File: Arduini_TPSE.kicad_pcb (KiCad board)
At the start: 2 copper layers, 26 x 57.5 mm, 27 parts, among them J1 2134441-2, J2 ICSP, P1 Digital, P2 Analog, SW1 SW_Push, U1 AMS1117-5.0, U2 FT232RL, U3 ATmega328-P, U4 AMS1117-3.3, Y1 16Mhz

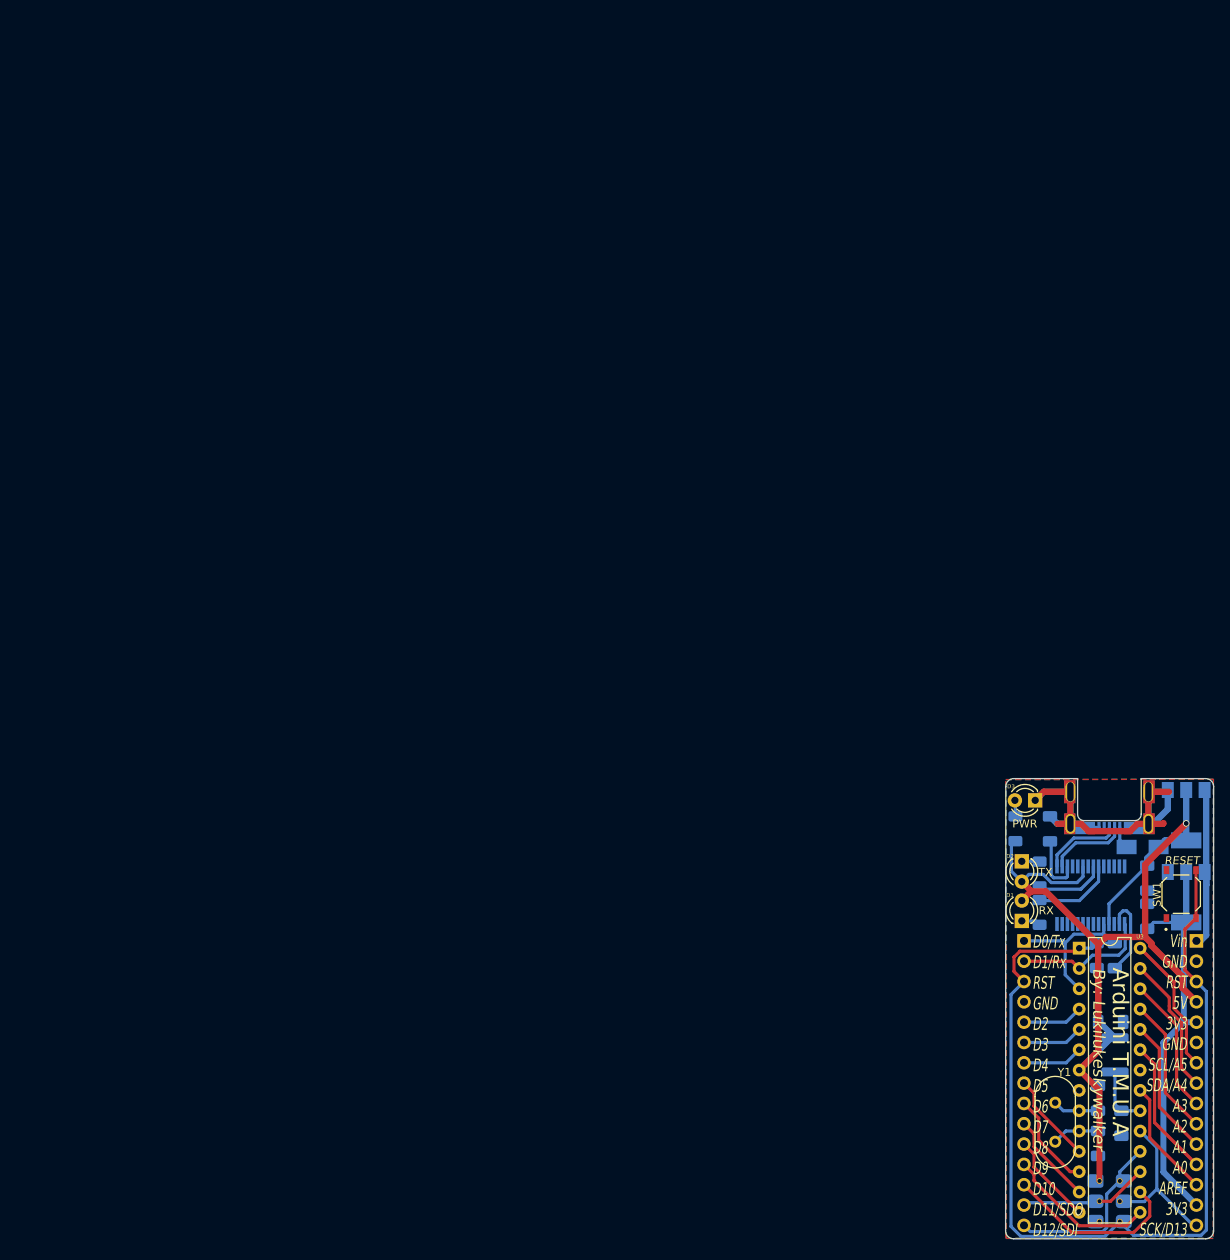
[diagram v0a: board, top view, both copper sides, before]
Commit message: Ampliacion
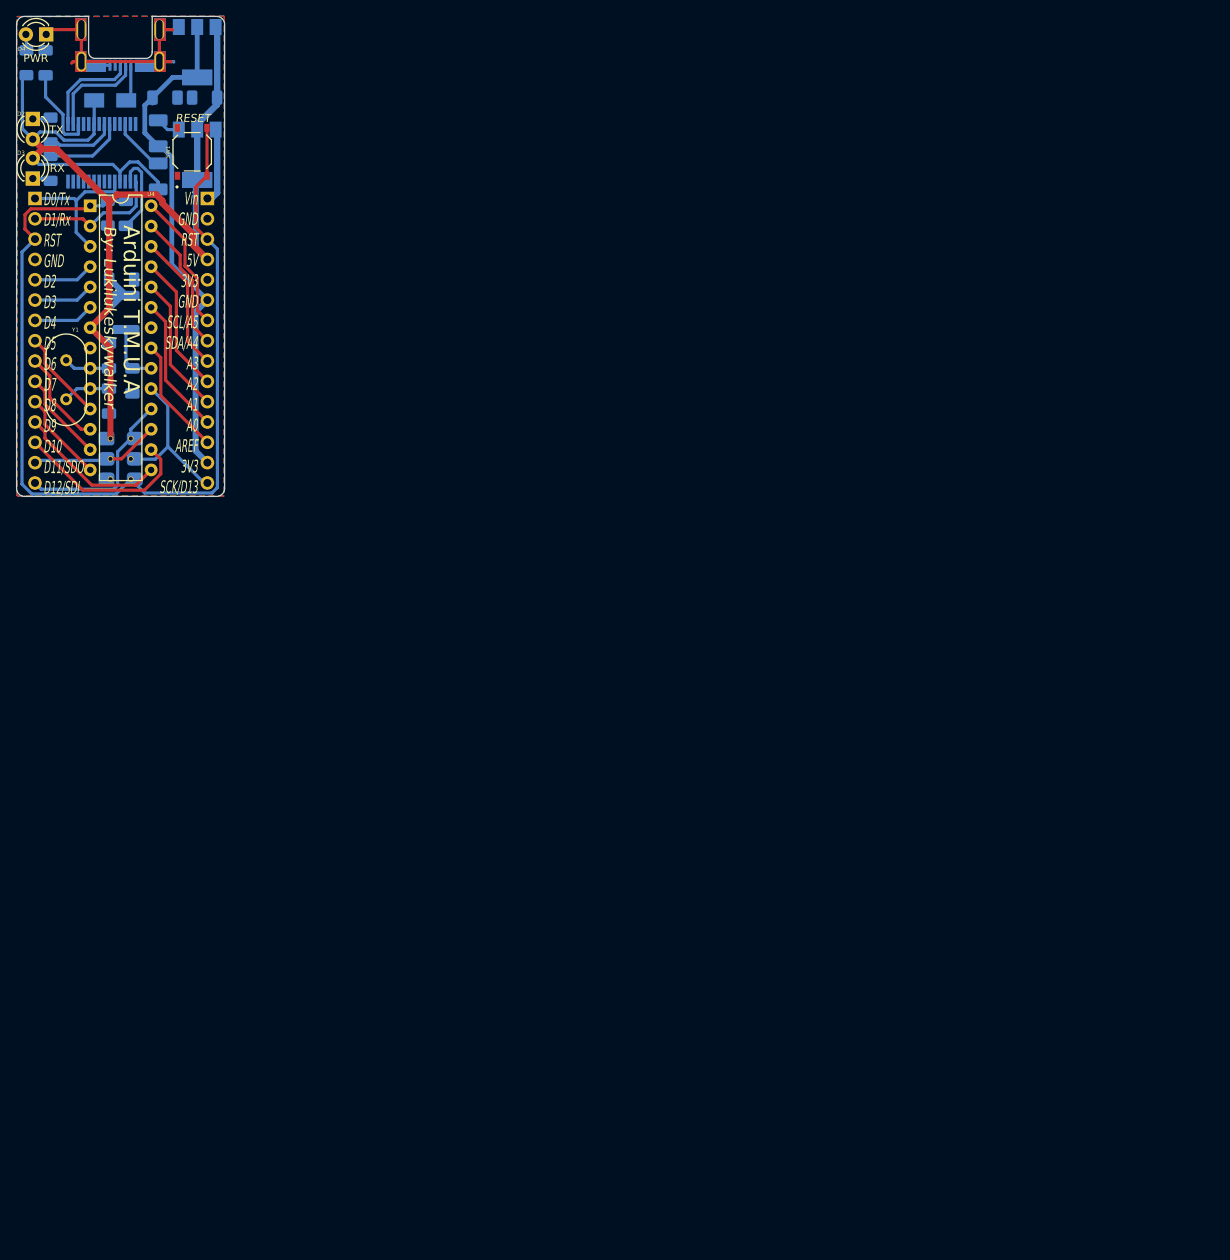
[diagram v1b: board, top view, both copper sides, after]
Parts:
- removed the D4 at (140.8, 43.8)
- added C10: 100n, Capacitor_SMD:C_1206_3216Metric_Pad1.33x1.80mm_HandSolder, B.Cu at (18.6, -49.9)
- added C8: 100n, Capacitor_SMD:C_1206_3216Metric_Pad1.33x1.80mm_HandSolder, B.Cu at (23.5, -49.9)
- added D1: D_Schottky, Diode_SMD:D_SMA, B.Cu at (11.7, -49.5)
- C7: footprint Capacitor_SMD:C_1206_3216Metric_Pad1.33x1.80mm_HandSolder -> Capacitor_Tantalum_SMD:CP_EIA-3528-15_AVX-H_Pad1.50x2.35mm_HandSolder
- C9: renamed from C8; footprint Capacitor_SMD:C_1206_3216Metric_Pad1.33x1.80mm_HandSolder -> Capacitor_Tantalum_SMD:CP_EIA-3528-15_AVX-H_Pad1.50x2.35mm_HandSolder
- moved U2 162.6 mm to (22.6, -55.5)
- moved C6 157.9 mm to (3.62, -54.2)
- moved C9 157.7 mm to (17.7, -45.4)
- moved D4 156.4 mm to (3.70, -57.8)
- moved R4 156.4 mm to (1.23, -54.2)
- moved J1 156.1 mm to (13.0, -58.4)
- moved R1 154.7 mm to (4.25, -41.0)
- moved R2 154.7 mm to (4.25, -45.8)
- moved C4 154.6 mm to (11.6, -17.6)
- moved C5 154.6 mm to (11.6, -11.9)
- moved L1 154.6 mm to (13.7, -23.0)
- moved C1 154.6 mm to (13.7, -35.4)
- moved C2 154.6 mm to (14.5, -14.4)
- moved C3 154.6 mm to (13.1, -27.1)
- moved D2 154.6 mm to (2.02, -47.2)
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- renumbered D1 to D3, D3 to D4, U4 to U2, U2 to U3, U3 to U4
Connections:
- P2 pad 5: +3V3 -> GND
- P2 pad 6: GND -> +3V3
- U2 pad 3: /Vin -> +5V
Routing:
- net +5V: track 133.8 -> 152.9 mm, vias 1 -> 0
- net +3V3: track 51.3 -> 65.4 mm
- net GND: track 58.2 -> 44.9 mm
- net /Vin: track 21.7 -> 9.50 mm
- net /3V3OUT: track 7.77 -> 11.3 mm
- net /D+: track 9.96 -> 12.5 mm
- net /D-: track 9.96 -> 12.5 mm
- net Net-(J1-Pad1): track 2.80 -> 4.64 mm
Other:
- board size 26 x 57.5 mm -> 26 x 60 mm
